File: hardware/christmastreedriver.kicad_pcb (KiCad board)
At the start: 4 copper layers, 38 x 25 mm, 57 parts, among them J1 M8S-03PMMR-SF8001, J2 USB4105, Q1 STL9P3LLH6, Q2 BC817RAPNZ, SW1 EVQPUC, SW2 EVQPUC, U1 STUSB4500QTR, U2 MAXM17630AME+ (3.3V), U3 CP2102N-A02-GQFN28R, U4 ESP32-PICO-D4, U5 DRV8244S

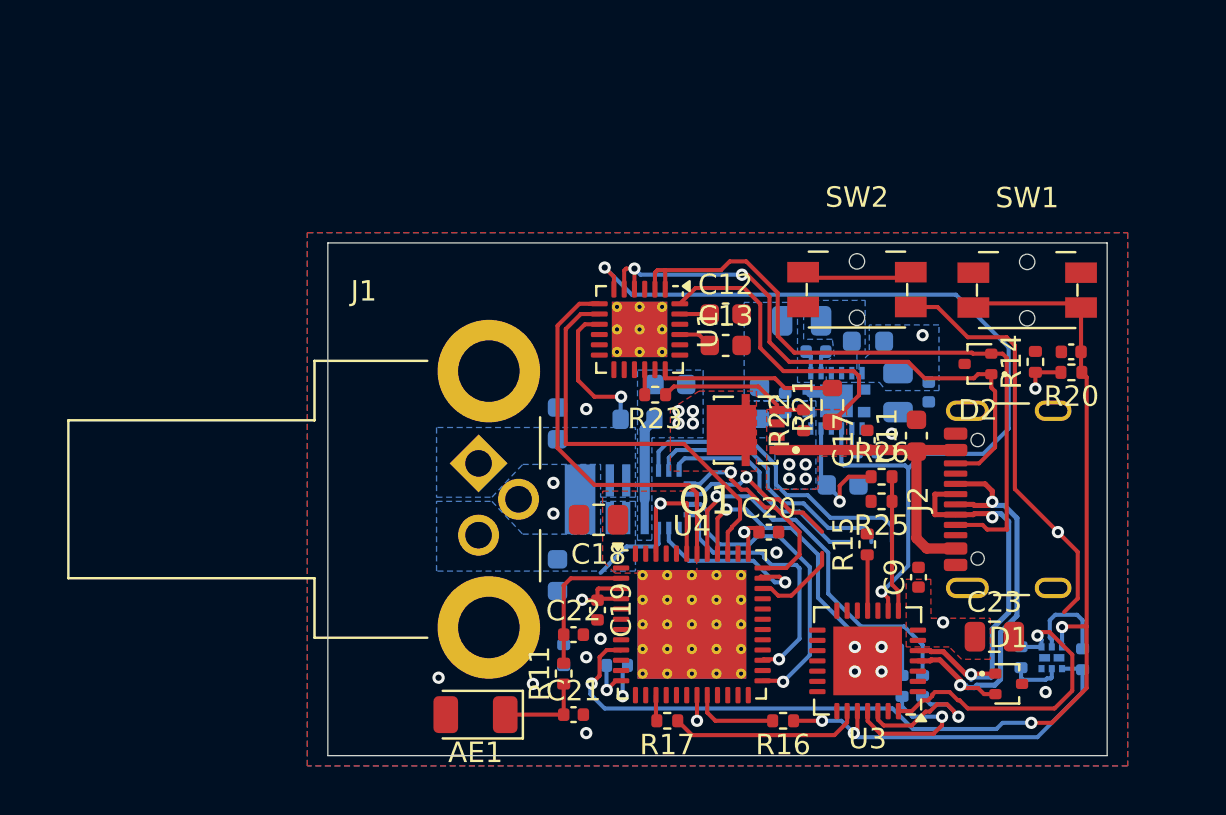
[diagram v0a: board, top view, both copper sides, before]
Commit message: Generated first bom
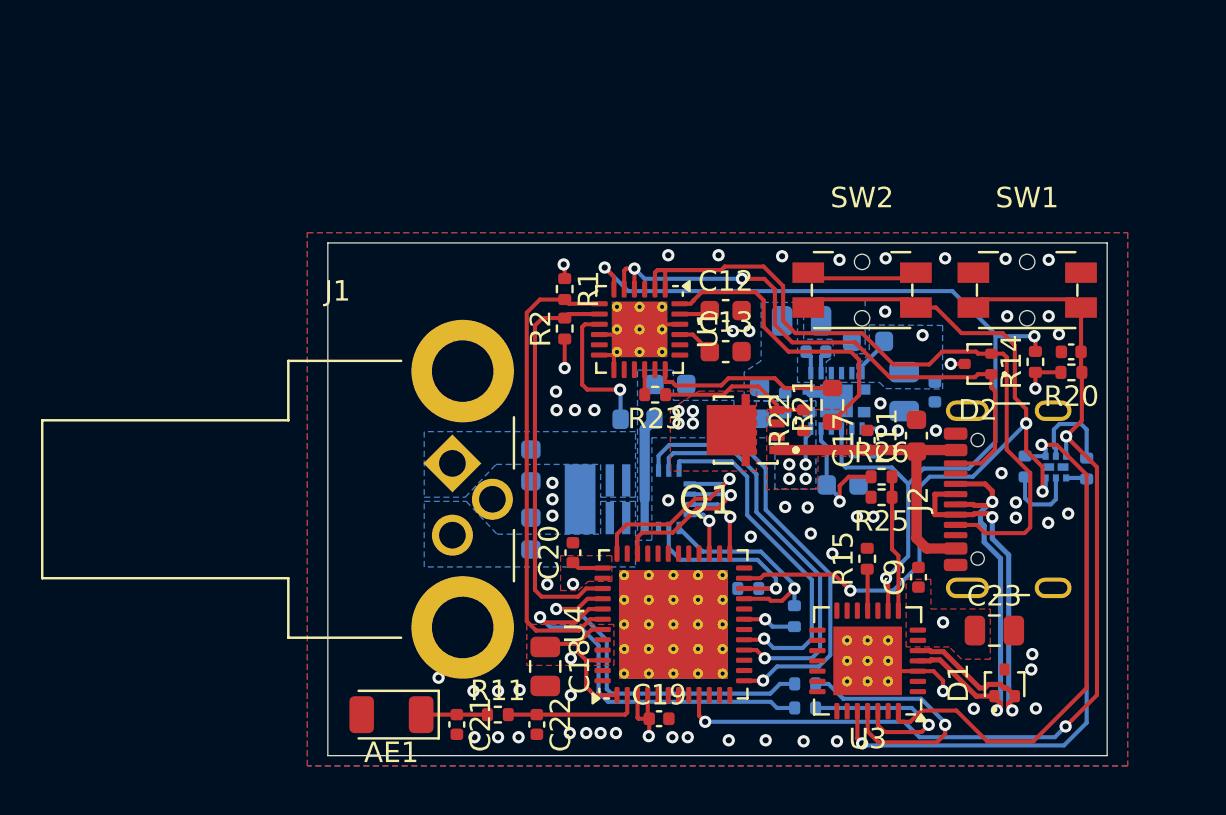
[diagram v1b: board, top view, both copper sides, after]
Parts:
- removed R16, R17: 0, Resistor_SMD:R_0402_1005Metric
- added R1: 2k, Resistor_SMD:R_0402_1005Metric, F.Cu at (146.6, 39.8)
- added R2: 2k, Resistor_SMD:R_0402_1005Metric, F.Cu at (146.6, 41.7)
- U3: footprint Package_DFN_QFN:QFN-28-1EP_5x5mm_P0.5mm_EP3.35x3.35mm -> Package_DFN_QFN:QFN-28-1EP_5x5mm_P0.5mm_EP3.35x3.35mm_ThermalVias
- moved C20 9.60 mm to (146.9, 52.6), turned to 90 degrees
- moved R10 9.57 mm to (155.5, 54.4), turned to 180 degrees
- moved R12 9.30 mm to (169.0, 48.4)
- moved Q2 9.30 mm to (170.5, 48.4)
- moved R13 9.30 mm to (172.0, 48.5)
- moved R9 8.98 mm to (157.8, 55.7), turned to 90 degrees
- moved C18 7.61 mm to (145.6, 58.1), turned to -90 degrees
- moved C19 6.09 mm to (151.2, 60.7), turned to 0 degrees
- moved R18 5.83 mm to (158.3, 60.2), turned to 180 degrees
- moved C21 5.71 mm to (141.3, 61.0), turned to -90 degrees
- moved C22 4.73 mm to (145.2, 61.0), turned to -90 degrees
- moved R19 4.73 mm to (158.3, 59.0), turned to 180 degrees
- moved AE1 4.10 mm to (138.1, 60.5)
- moved R11 3.78 mm to (143.3, 60.5), turned to 0 degrees
- moved C15 2.43 mm to (144.9, 48.4), turned to -90 degrees
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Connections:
- D1 pad 1: /Microcontroller/USB_D- -> /Microcontroller/USB_D+
- D1 pad 2: /Microcontroller/USB_D+ -> /Microcontroller/USB_D-
- U4 pad 10: /Bridge Driver/_EN/IN1 -> unconnected-(U4-IO34-Pad10)
- U4 pad 11: /Bridge Driver/_PH/IN2 -> unconnected-(U4-IO35-Pad11)
- U4 pad 12: /Bridge Driver/nFAULT -> unconnected-(U4-IO32-Pad12)
- U4 pad 16: unconnected-(U4-IO27-Pad16) -> /Bridge Driver/_EN/IN1
- U4 pad 17: unconnected-(U4-IO14-Pad17) -> /Bridge Driver/_PH/IN2
- U4 pad 21: unconnected-(U4-IO15-Pad21) -> /Bridge Driver/nFAULT
- U4 pad 22: unconnected-(U4-IO2-Pad22) -> /Bridge Driver/Current Sense
- U4 pad 35: /Bridge Driver/Current Sense -> unconnected-(U4-IO18-Pad35)
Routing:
- net +3.3V: track 72.2 -> 96.2 mm, vias 8 -> 9
- net /Microcontroller/IO0: track 20.4 -> 39.3 mm, vias 1 -> 3
- net GND: track 5.48 -> 17.5 mm, vias 14 -> 63
- net /Microcontroller/~{DTR}: track 15.2 -> 26.4 mm
- net /SPI_MOSI: track 15.2 -> 4.03 mm
- net /SPI_MISO: track 12.7 -> 2.67 mm
- net /Microcontroller/~{CTS}: track 9.36 -> 0.00 mm
- net /Bridge Driver/nFAULT: track 2.09 -> 10.5 mm
- net /Microcontroller/~{RTS}: track 18.6 -> 26.0 mm, vias 2 -> 1
- net /Microcontroller/EN: track 55.2 -> 48.1 mm
- net /Bridge Driver/_DRVOFF: track 15.5 -> 21.8 mm, vias 0 -> 1
- net /Bridge Driver/_EN/IN1: track 13.3 -> 19.3 mm, vias 0 -> 1
- net /Bridge Driver/_PH/IN2: track 11.0 -> 17.0 mm, vias 0 -> 1
- net /Microcontroller/RXD: track 7.60 -> 12.8 mm
- net /Microcontroller/_~{RTS}: track 4.21 -> 0.00 mm
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
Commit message: Flipped some stuff
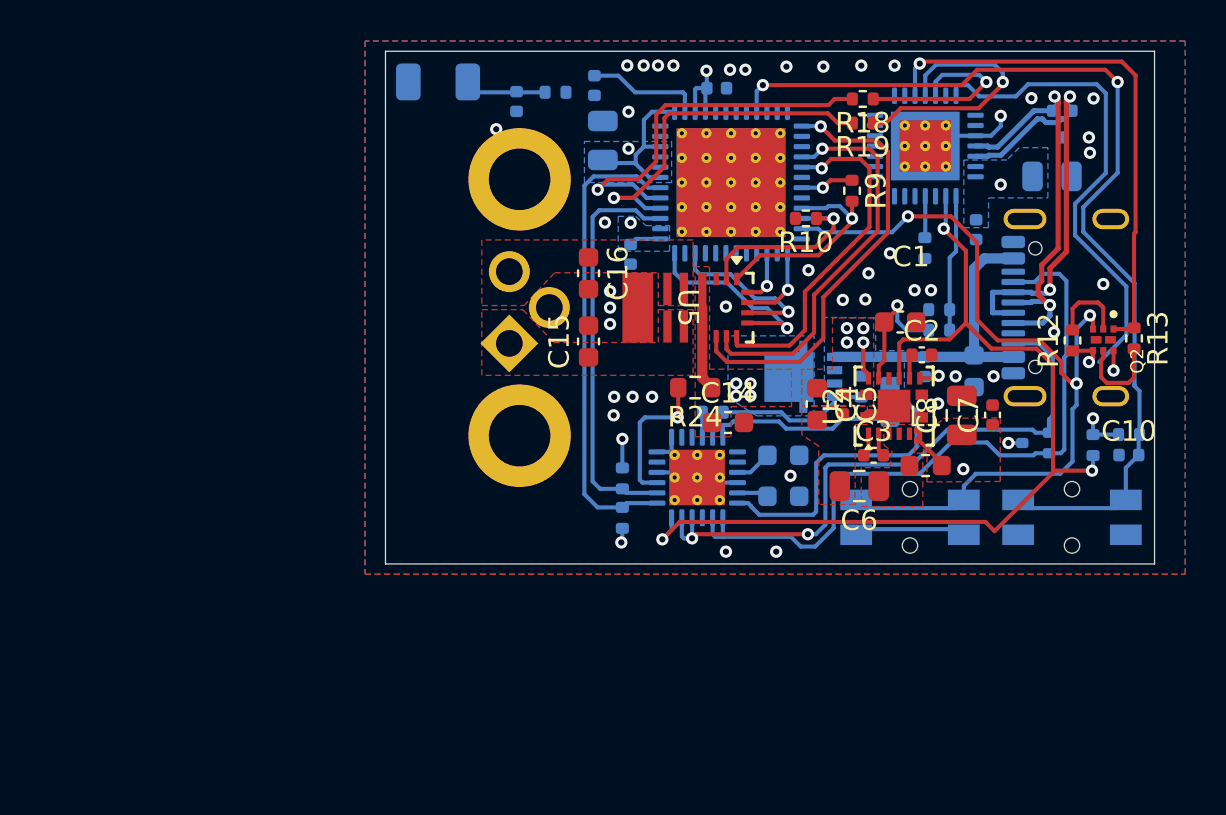
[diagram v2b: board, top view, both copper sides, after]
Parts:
- AE1, C10, C11, C12, C13, C17, C18, C19, C20, C21, C22, C23, C9, D1, D2, J1, J2, Q1, R1, R11, R14, R15, R2, R20, R21, R22, R23, R25, R26, SW1, SW2, U1, U3, U4: moved to B.Cu
- C1, C14, C15, C16, C2, C3, C4, C5, C6, C7, C8, L1, NT1, Q2, R10, R12, R13, R18, R19, R24, R9, U2, U5: moved to F.Cu
- moved C22 31.3 mm to (148.0, 29.8)
- moved AE1 30.9 mm to (140.4, 29.6)
- moved C19 30.9 mm to (154.0, 30.0)
- moved C21 30.5 mm to (144.2, 30.6)
- moved R11 30.5 mm to (146.1, 30.2)
- moved R18 29.8 mm to (161.1, 30.5)
- moved R19 27.5 mm to (161.1, 31.7)
- moved D1 27.4 mm to (170.8, 31.7), turned to -90 degrees
- moved C18 25.8 mm to (148.4, 32.5), turned to 90 degrees
- moved U3 25.3 mm to (164.1, 32.8)
- moved C23 22.3 mm to (170.3, 34.3)
- moved U4 21.7 mm to (154.7, 34.6), turned to -90 degrees
- moved R9 20.9 mm to (160.6, 35.0), turned to -90 degrees
- moved R10 18.3 mm to (158.3, 36.3)
- moved C9 17.2 mm to (166.6, 36.9), turned to -90 degrees
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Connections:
- J1 pad 1: /Bridge Driver/A -> /Bridge Driver/B
- J1 pad 3: /Bridge Driver/B -> /Bridge Driver/A
- U1 pad 11: unconnected-(U1-ATTACH-Pad11) -> /Microcontroller/PD_Attach
- U1 pad 19: unconnected-(U1-ALERT-Pad19) -> /Microcontroller/PD_Reset
- U1 pad 6: /Microcontroller/Reset -> /Microcontroller/PD_Alert
- U4 pad 12: unconnected-(U4-IO32-Pad12) -> /Microcontroller/PD_Attach
- U4 pad 35: unconnected-(U4-IO18-Pad35) -> /Microcontroller/PD_Alert
- U4 pad 38: unconnected-(U4-IO19-Pad38) -> /Microcontroller/PD_Reset
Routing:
- net /Microcontroller/LNA_IN: track 6.69 -> 5.64 mm
- net /Microcontroller/~{DTR}: track 26.4 -> 25.4 mm
- net /USB PD/CC1: track 35.1 -> 34.3 mm
- net /Microcontroller/Antenna_50R: track 3.33 -> 4.08 mm
- net /Microcontroller/IO0: track 39.3 -> 40.0 mm
- net VBUS: track 31.6 -> 32.2 mm
- net /USB PD/CC2: track 29.1 -> 29.7 mm
- net GND: vias 63 -> 43
- added copper zone on F.Cu, net /Bridge Driver/A
- added copper zone on F.Cu, net /Bridge Driver/B
- added copper zone on F.Cu, net /Power Supply/_3V3
- added copper zone on F.Cu, net GNDPWR
- removed copper zone on B.Cu, net /Bridge Driver/A
- removed copper zone on B.Cu, net /Bridge Driver/B
- removed copper zone on B.Cu, net /Power Supply/_3V3
- removed copper zone on B.Cu, net GNDPWR
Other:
- board size 38 x 25 mm -> 37.5 x 25 mm
